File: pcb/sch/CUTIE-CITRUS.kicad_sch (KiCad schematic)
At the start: 0 parts

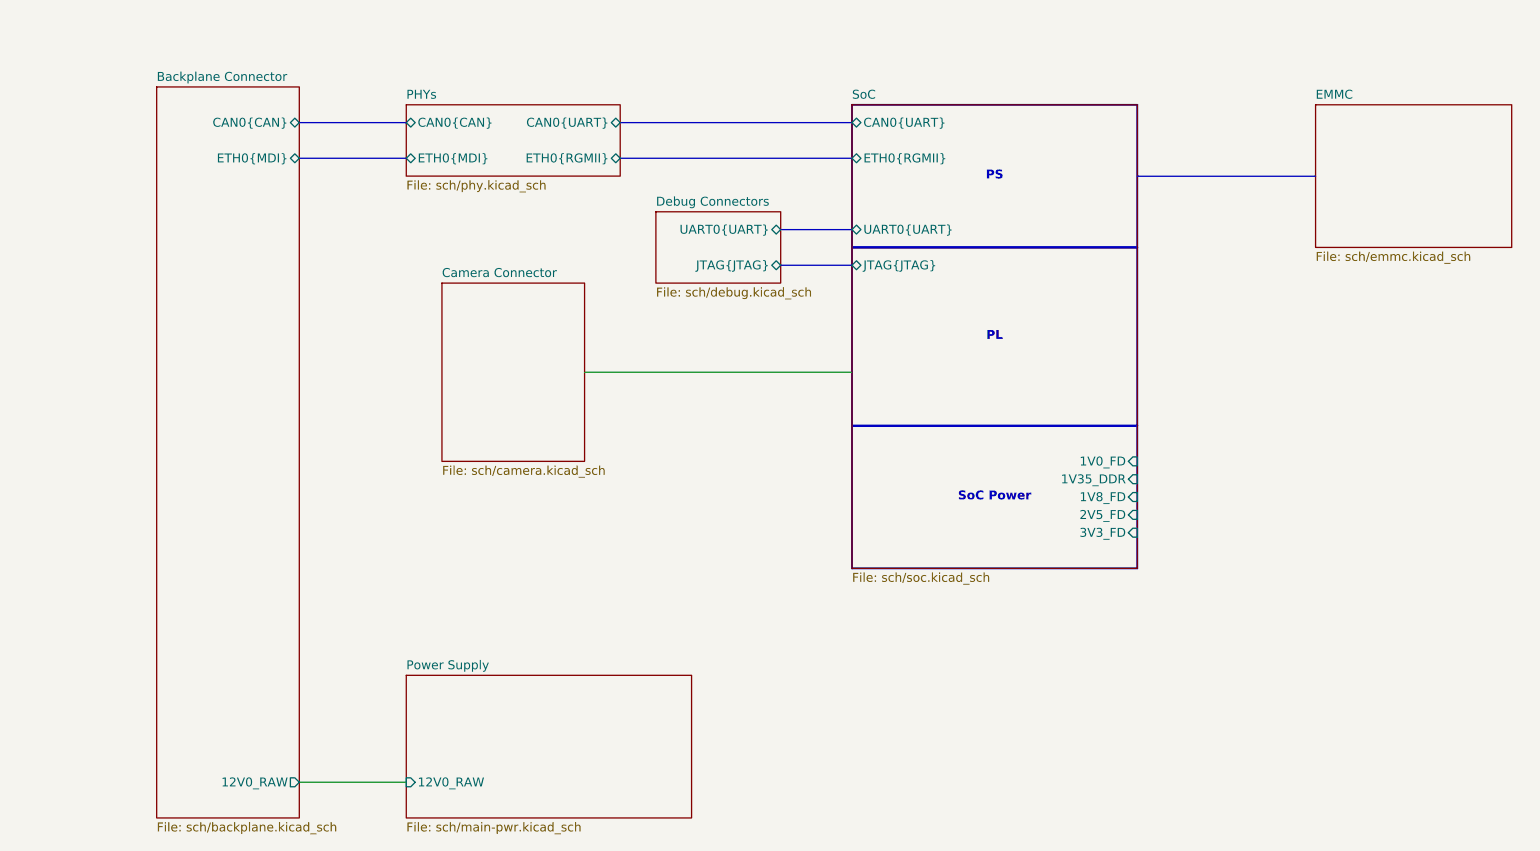
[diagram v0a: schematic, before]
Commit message: more pin definition pending define for how boot mode and power cycling will work, potential uc (stm32)
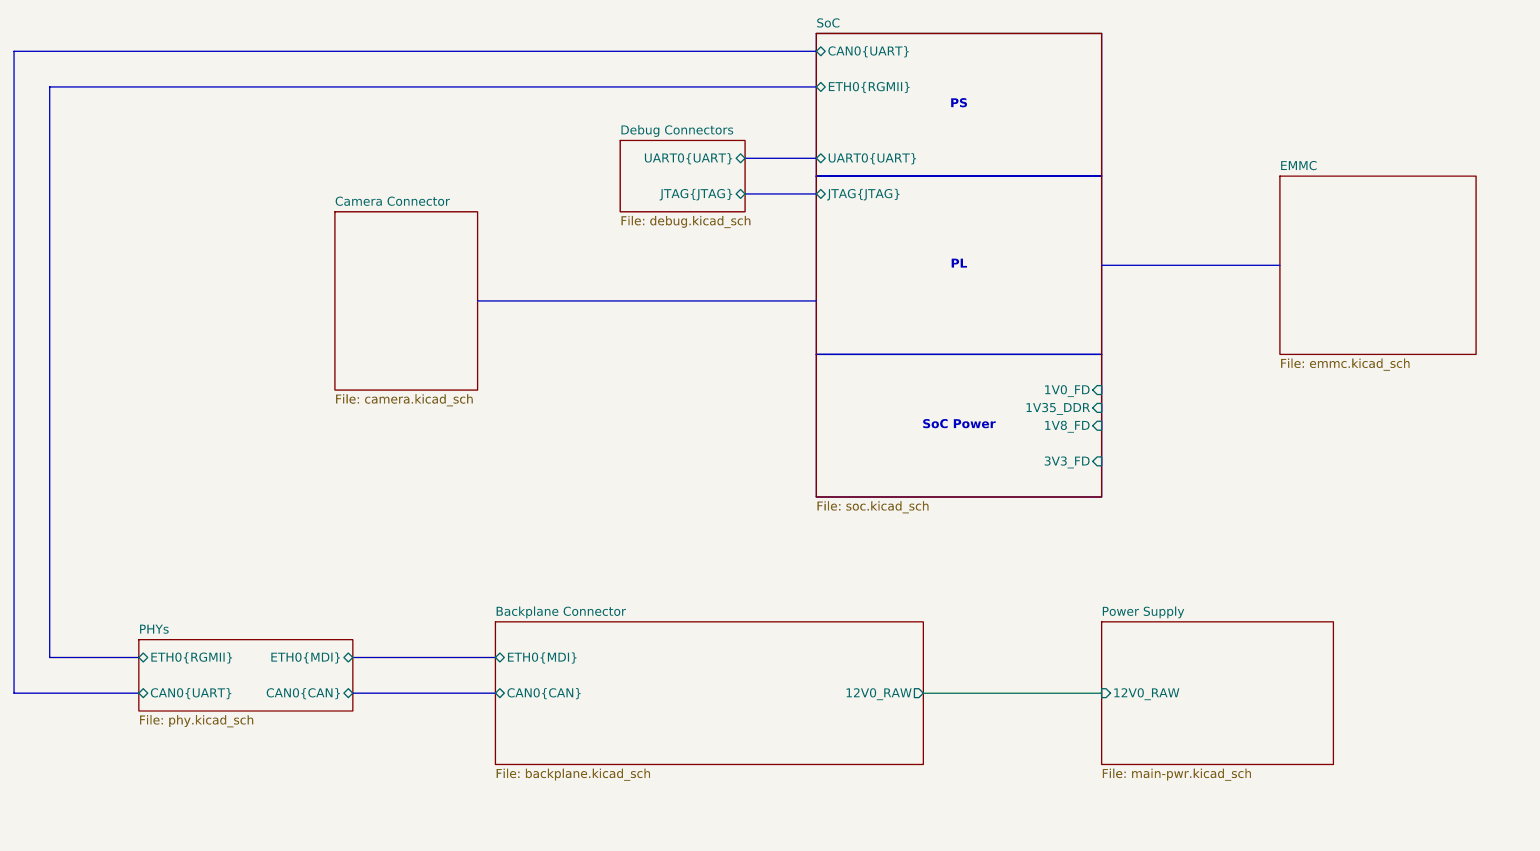
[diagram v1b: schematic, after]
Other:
- sheet Backplane Connector: file sch/backplane.kicad_sch -> backplane.kicad_sch
- sheet Camera Connector: file sch/camera.kicad_sch -> camera.kicad_sch
- sheet Debug Connectors: file sch/debug.kicad_sch -> debug.kicad_sch
- sheet EMMC: file sch/emmc.kicad_sch -> emmc.kicad_sch
- sheet PHYs: file sch/phy.kicad_sch -> phy.kicad_sch
- sheet Power Supply: file sch/main-pwr.kicad_sch -> main-pwr.kicad_sch
- sheet SoC: file sch/soc.kicad_sch -> soc.kicad_sch
- sheet SoC ports: added none; removed 2V5_FD
